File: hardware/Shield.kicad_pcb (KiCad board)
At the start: 2 copper layers, 70.1 x 40.6 mm, 29 parts, among them IC1 TP4056-42-ESOP8, P1 CONN_14_1, P2 CONN_14_2, SW1 JS202011SCQN

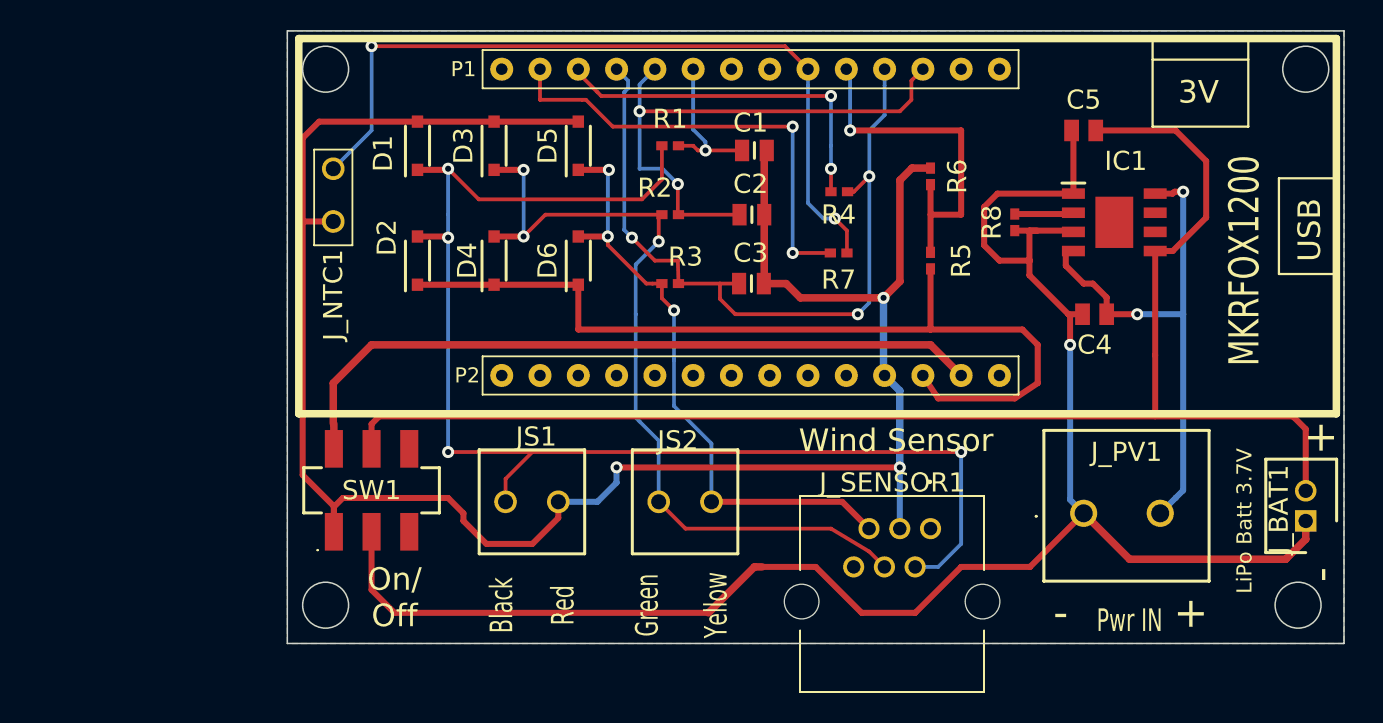
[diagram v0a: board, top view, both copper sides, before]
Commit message: reorg sockets
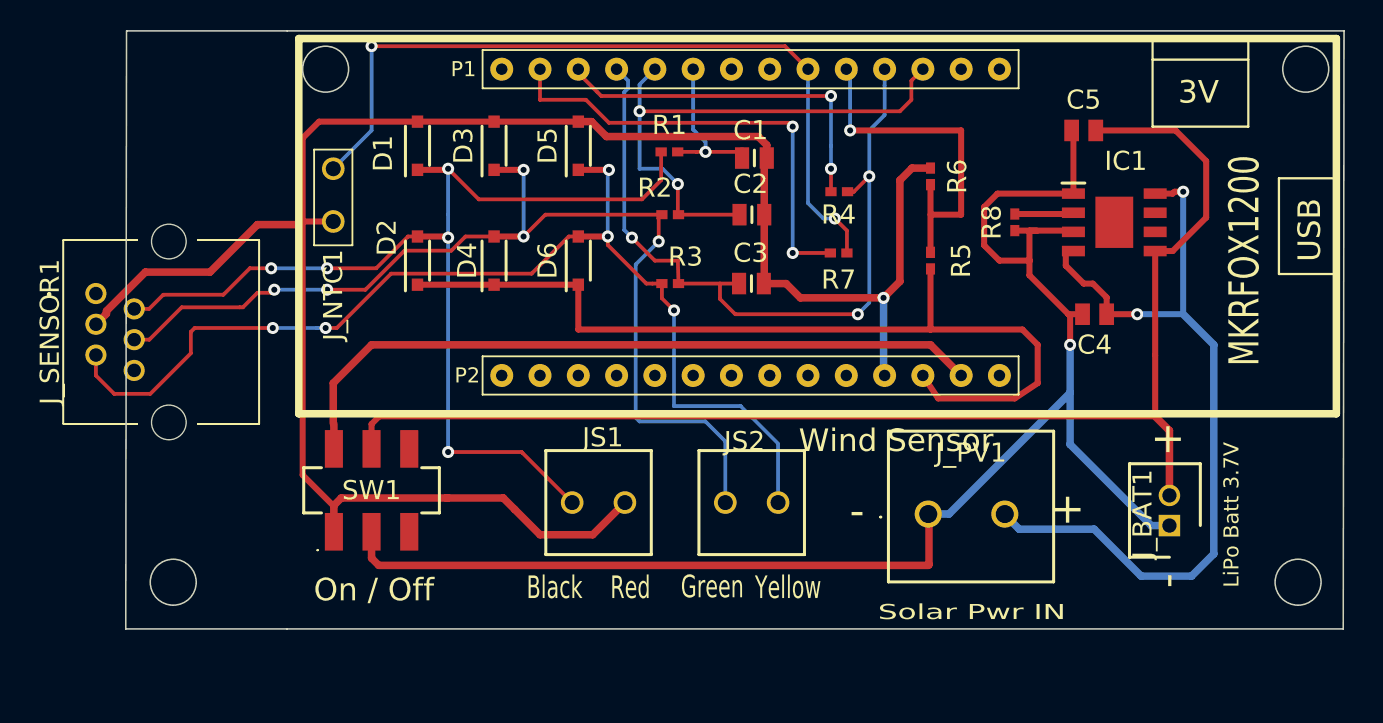
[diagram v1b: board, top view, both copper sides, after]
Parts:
- moved J_SENSOR1 57.5 mm to (62.0, 83.5), turned to 90 degrees
- moved J_PV1 10.3 mm to (117.2, 98.1)
- moved J_BAT1 9.05 mm to (133.2, 98.9)
- moved JS1 4.42 mm to (93.6, 97.3)
- moved JS2 4.42 mm to (103.7, 97.3)
- moved C1 0.50 mm to (105.7, 74.5)
- moved R1 0.41 mm to (100.0, 74.1)
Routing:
- net Wire4: track 40.7 -> 72.9 mm, vias 3 -> 5
- net VPV: track 34.6 -> 53.6 mm
- net Wire1: track 88.6 -> 70.7 mm, vias 4 -> 5
- net GND: track 116.0 -> 100.1 mm
- net Wire3: track 55.2 -> 69.8 mm, vias 3 -> 5
- net VBAT: track 95.5 -> 86.7 mm
- net MGND: track 135.7 -> 135.9 mm, vias 3 -> 1
- removed copper zone on B.Cu, net GND
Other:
- board size 70.1 x 40.6 mm -> 80.8 x 39.7 mm
- board text added: "MkrfoxWindShield v1.1"
- board text added: "On / Off"
- board text added: "Solar Pwr IN"
- board text removed: "MkrfoxWindShield v1.0"
- board text removed: "On/ Off"
- board text removed: "Pwr IN"
